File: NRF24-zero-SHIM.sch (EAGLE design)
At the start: 36 parts

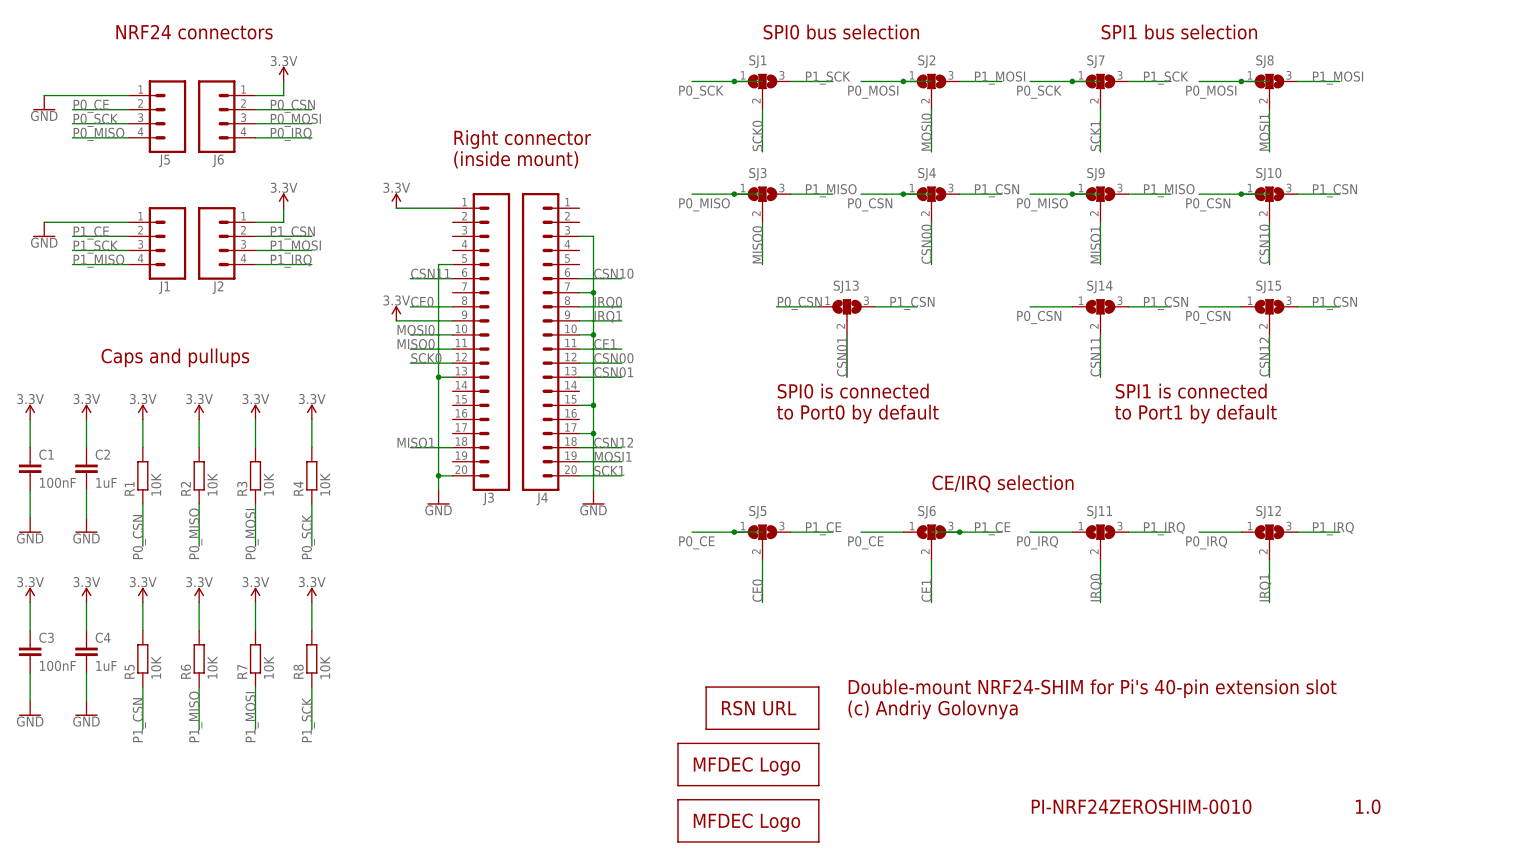
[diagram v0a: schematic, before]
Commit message: Added zero-sized board.
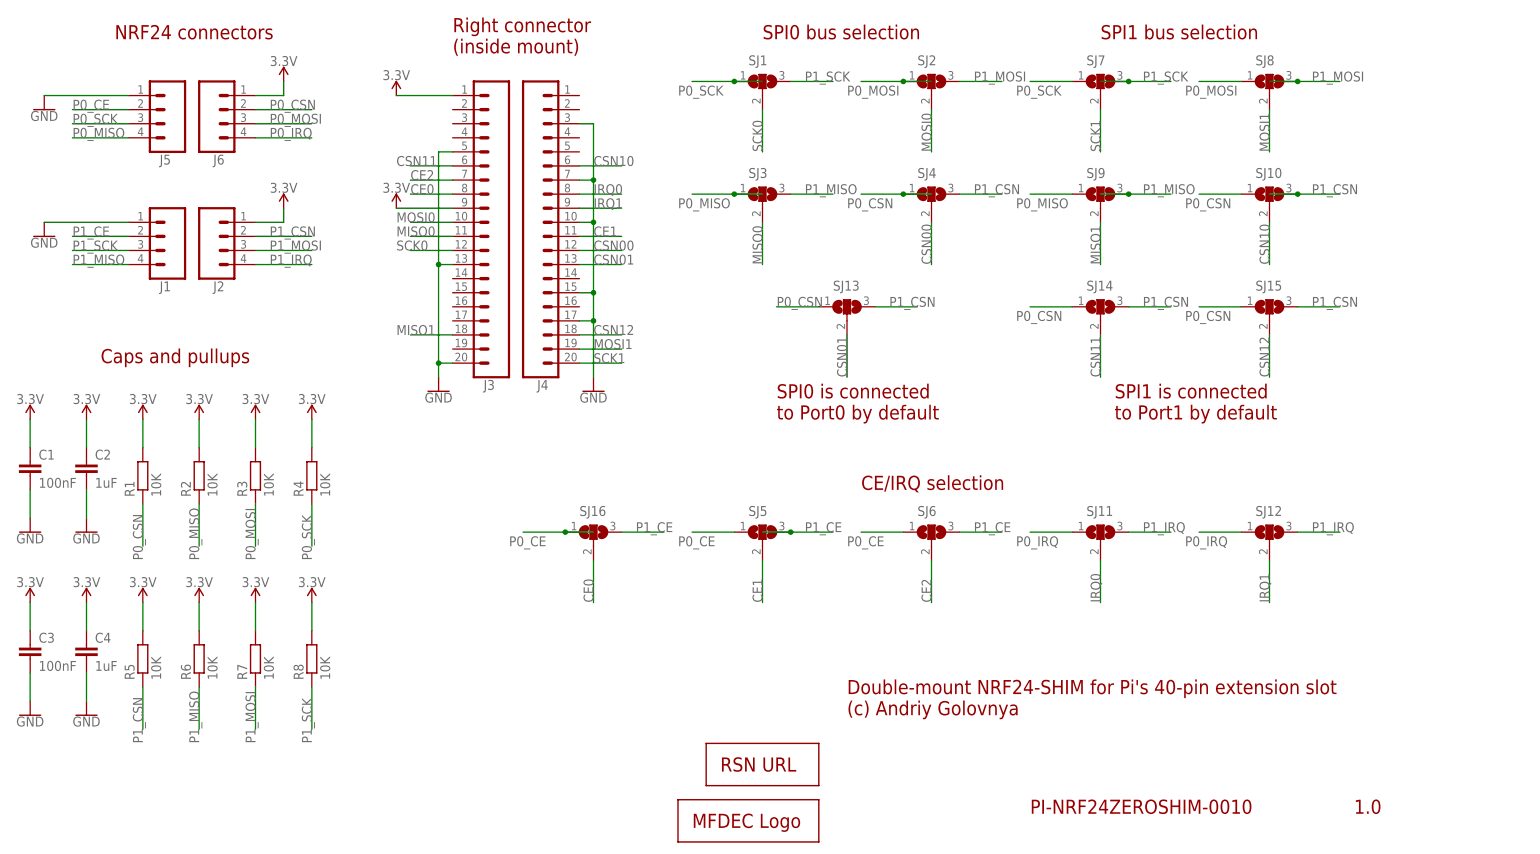
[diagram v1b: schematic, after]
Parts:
- removed LOGO2: MFDECLOGO_L_20MM, _my_logos:MFDECLOGO_L_20MM
- added SJ16: (no value), _my_jumpers:SJ2
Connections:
- new net CE2: J3.7, SJ6.2
- net CE0: now also SJ16.2; no longer SJ5.2
- net CE1: now also SJ5.2; no longer SJ6.2
- net P0_CE: now also SJ16.1
- net P1_CE: now also SJ16.3
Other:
- moved on the sheet: J3, J4
